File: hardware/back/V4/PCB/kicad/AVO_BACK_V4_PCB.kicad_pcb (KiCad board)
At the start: 4 copper layers, 46.7 x 47.4 mm, 81 parts, among them J1 USB-C 16P, J2 BATERÍA 1S, J3 microSD DM3AT, J4 URTK1.2 (8 hilos), P1 CONTACTO SYS, P2 CONTACTO BAT, P3 CONTACTO GND, Q3 AO3401A, Q4 AO3401A, U2 BQ24072RGTR, U3 TLV75733PDBVR, U4 ESP32-S3-MINI-1U-N8, U6 USBLC6-2SC6, U7 RT9080-33GJ5

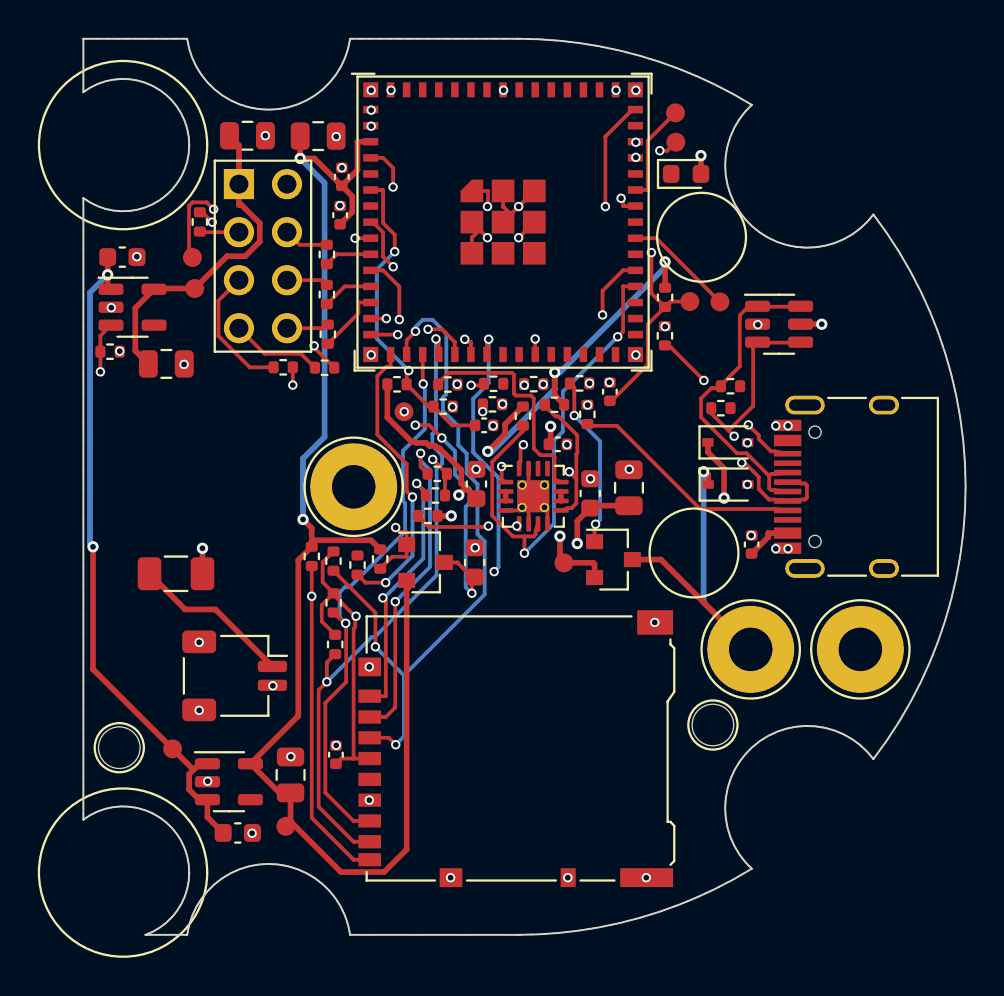
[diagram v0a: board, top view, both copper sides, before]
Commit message: PCB espalda V4: resultados de KiCad 9 de c1e0e26 (puerta: true) [skip ci]
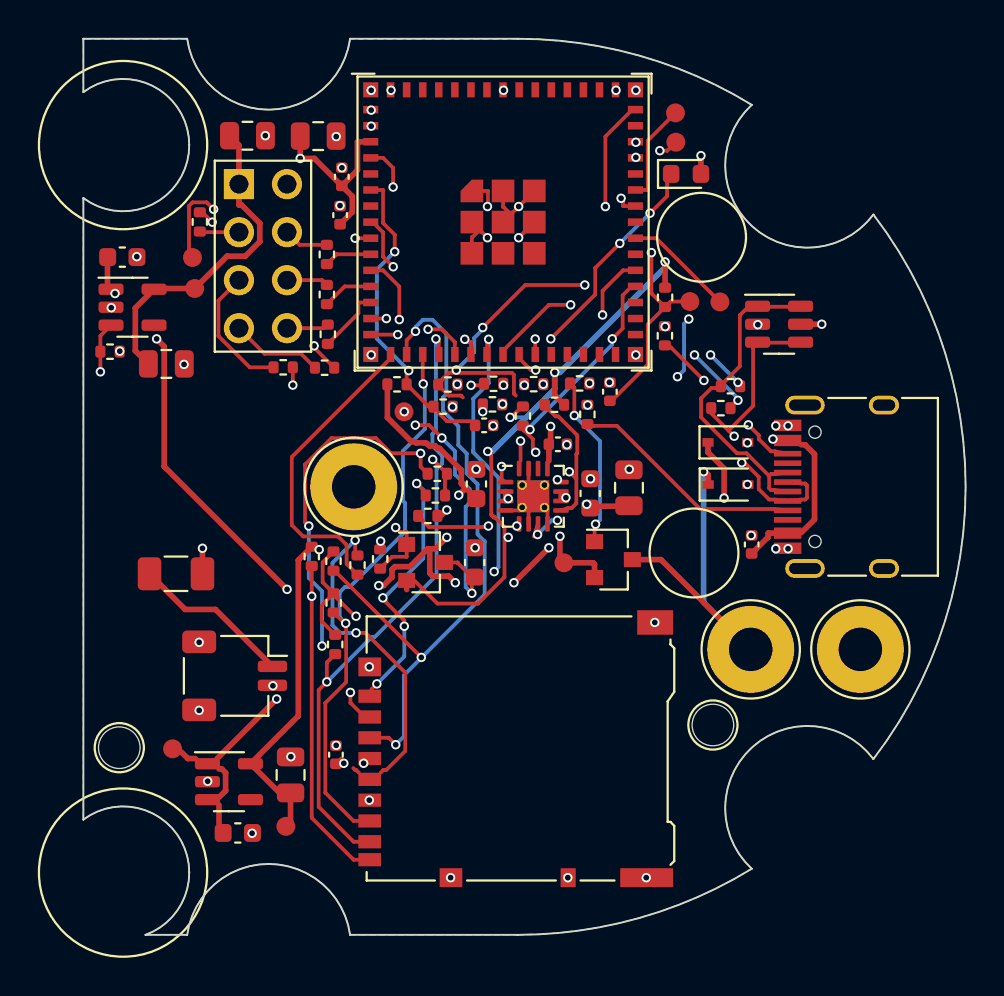
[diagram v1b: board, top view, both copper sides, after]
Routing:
- net +3V3: track 124.8 -> 99.8 mm, vias 6 -> 9
- net CHG_ILIM: track 12.0 -> 34.8 mm, vias 0 -> 6
- net SD_CLK: track 0.00 -> 16.8 mm, vias 0 -> 2
- net USB_DP: track 0.00 -> 16.6 mm, vias 0 -> 3
- net USB_DM: track 0.00 -> 15.5 mm, vias 0 -> 3
- net LED_K: track 0.00 -> 14.4 mm, vias 0 -> 4
- net VBUS: track 21.7 -> 31.8 mm, vias 2 -> 3
- net CHG_PG: track 26.8 -> 18.1 mm, vias 2 -> 5
- net VSYS: track 68.6 -> 61.3 mm, vias 4 -> 12
- net SD_D3: track 25.2 -> 30.5 mm, vias 3 -> 5
- net SD_CMD: track 37.0 -> 36.1 mm
- net BAT_ADC: track 16.8 -> 16.1 mm
- net +3V3_SD: track 42.2 -> 42.6 mm, vias 5 -> 7
- net SD_D2: track 25.8 -> 25.7 mm, vias 3 -> 5
- net VBAT: vias 2 -> 3
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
